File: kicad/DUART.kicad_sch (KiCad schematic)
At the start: 1 part

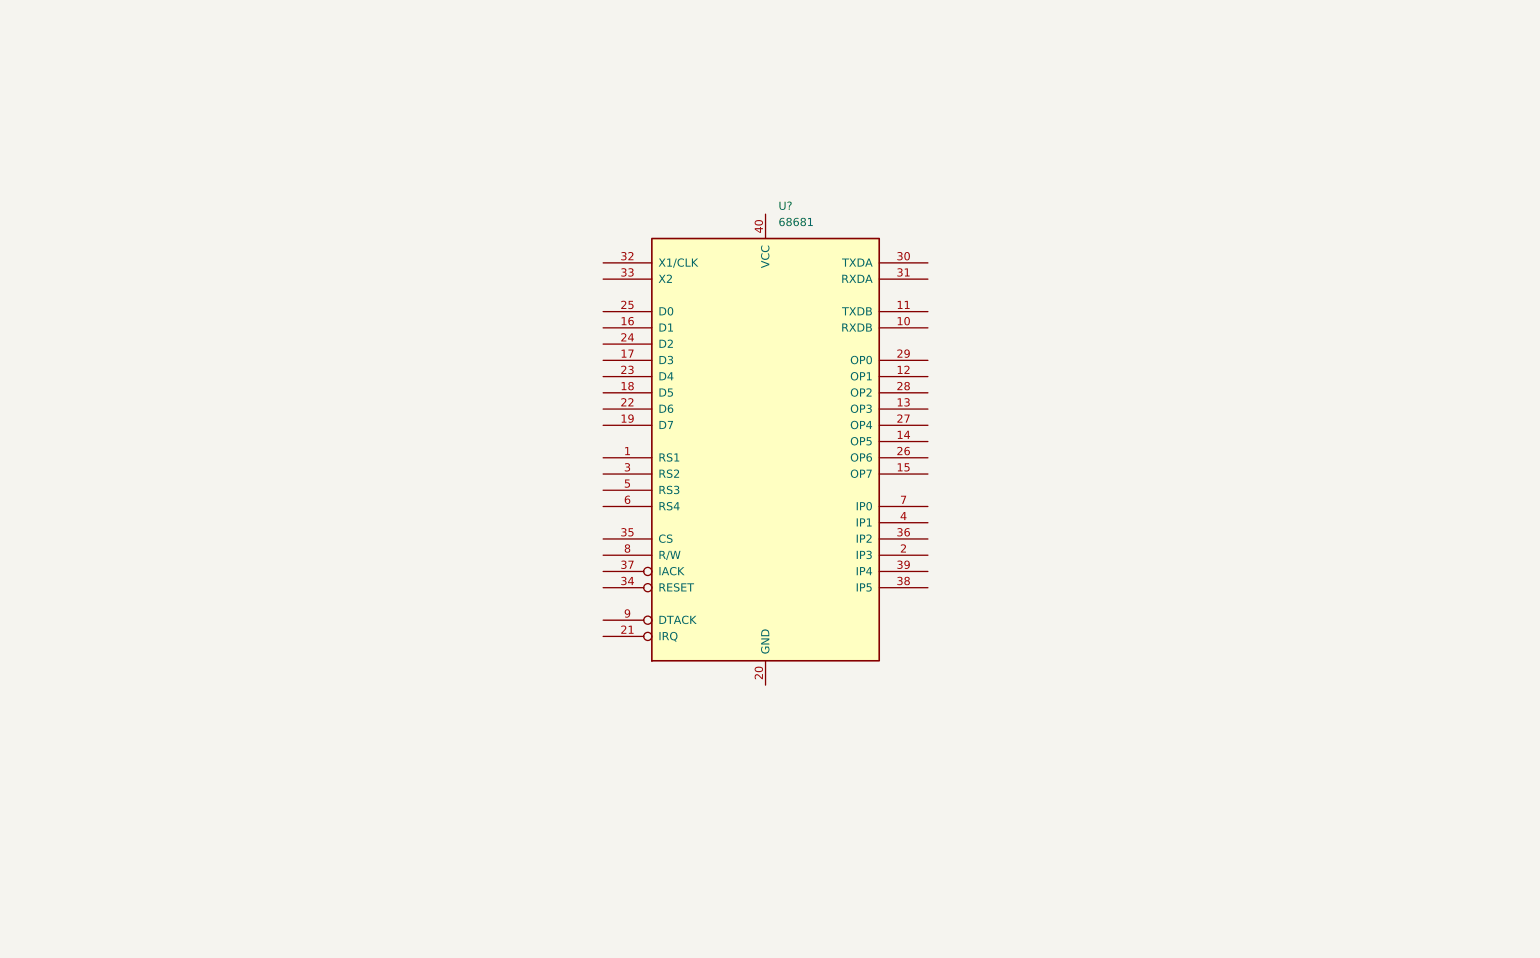
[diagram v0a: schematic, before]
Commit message: Lot of stuff. Memmory decoder in GAL Added README for Digital Updated sketch for Arduino
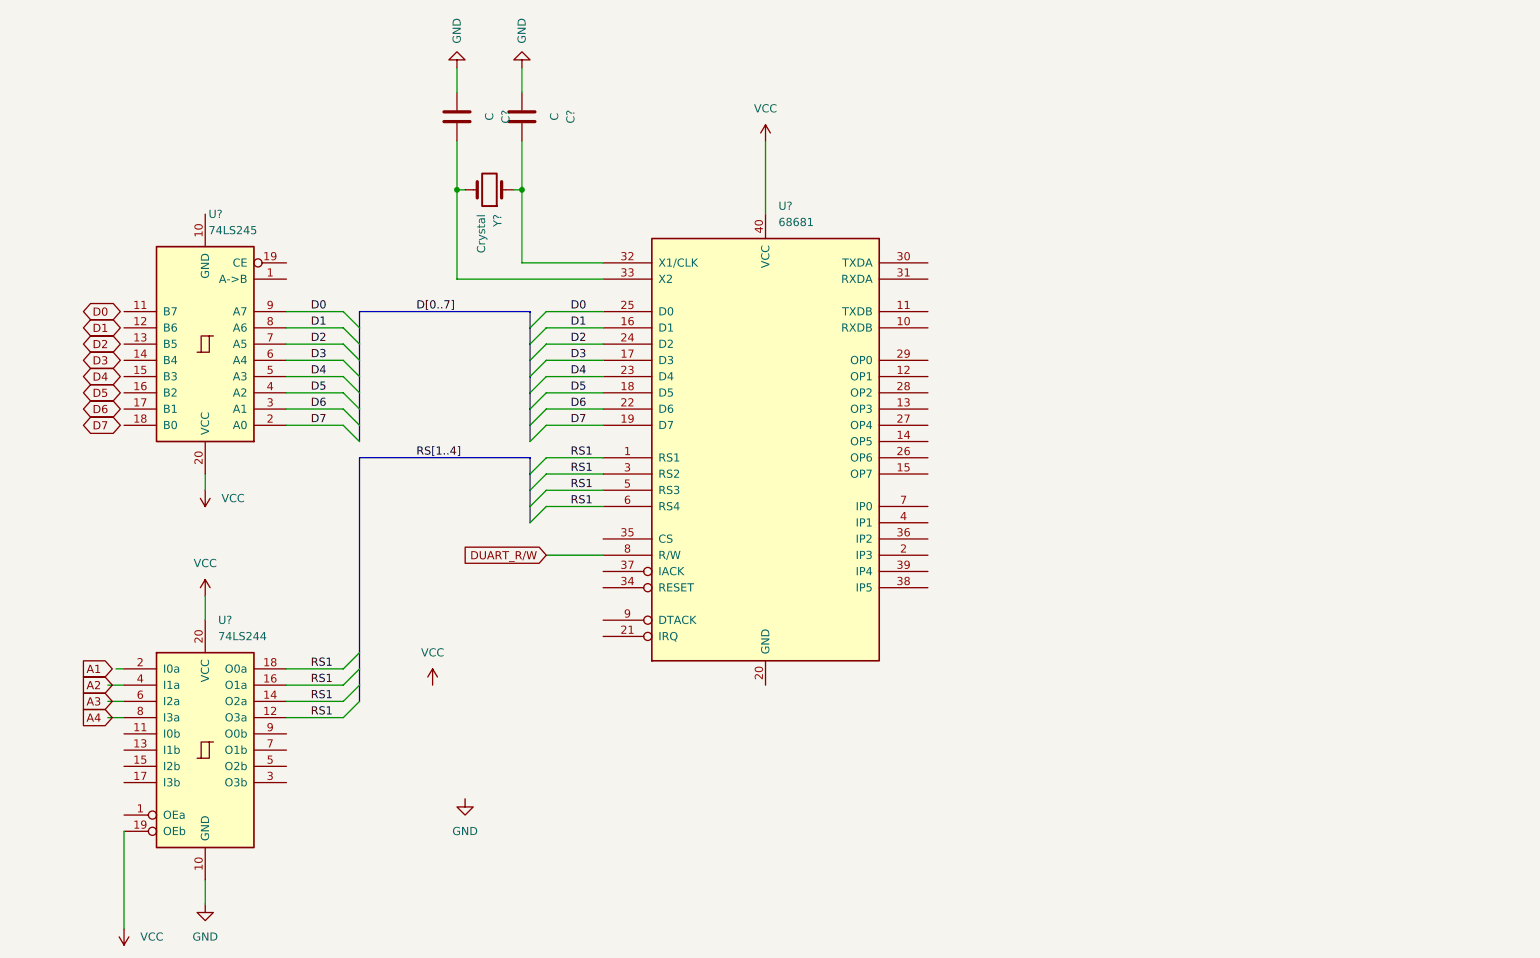
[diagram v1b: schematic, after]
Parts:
- added C? (x2): C, symbol Device:C
- added U?: 74LS245, symbol 74xx:74LS245
- added U?: 74LS244, symbol 74xx:74LS244
- added Y?: Crystal, symbol Device:Crystal
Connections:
- net RS1: now reaches U?.1 (RS1)
- net RS1: now also U?.3 (RS2), U?.5 (RS3), U?.6 (RS4), U?.12 (O3a), U?.14 (O2a), U?.16 (O1a), U?.18 (O0a)
- net D1: now reaches U?.16 (D1)
- net D1: now also U?.8 (A6)
- net D3: now reaches U?.17 (D3)
- net D3: now also U?.6 (A4)
- net D5: now reaches U?.18 (D5)
- net D5: now also U?.4 (A2)
- net D7: now reaches U?.19 (D7)
- net D7: now also U?.2 (A0)
- net D6: now reaches U?.22 (D6)
- net D6: now also U?.3 (A1)
- net D4: now reaches U?.23 (D4)
- net D4: now also U?.5 (A3)
- net D2: now reaches U?.24 (D2)
- net D2: now also U?.7 (A5)
- net D0: now reaches U?.25 (D0)
- net D0: now also U?.9 (A7)
- net at U?.32 (X1/CLK): now also C?.2, Y?.1
- net at U?.33 (X2): now also C?.2, Y?.2
- net VCC: now reaches U?.40 (VCC)
- net VCC: now also U?.19 (OEb), U?.20 (VCC), U?.20 (VCC)
- net DUART_R/W: now reaches U?.8 (R/W)
- new net GND: C?.1, C?.1, U?.10 (GND)

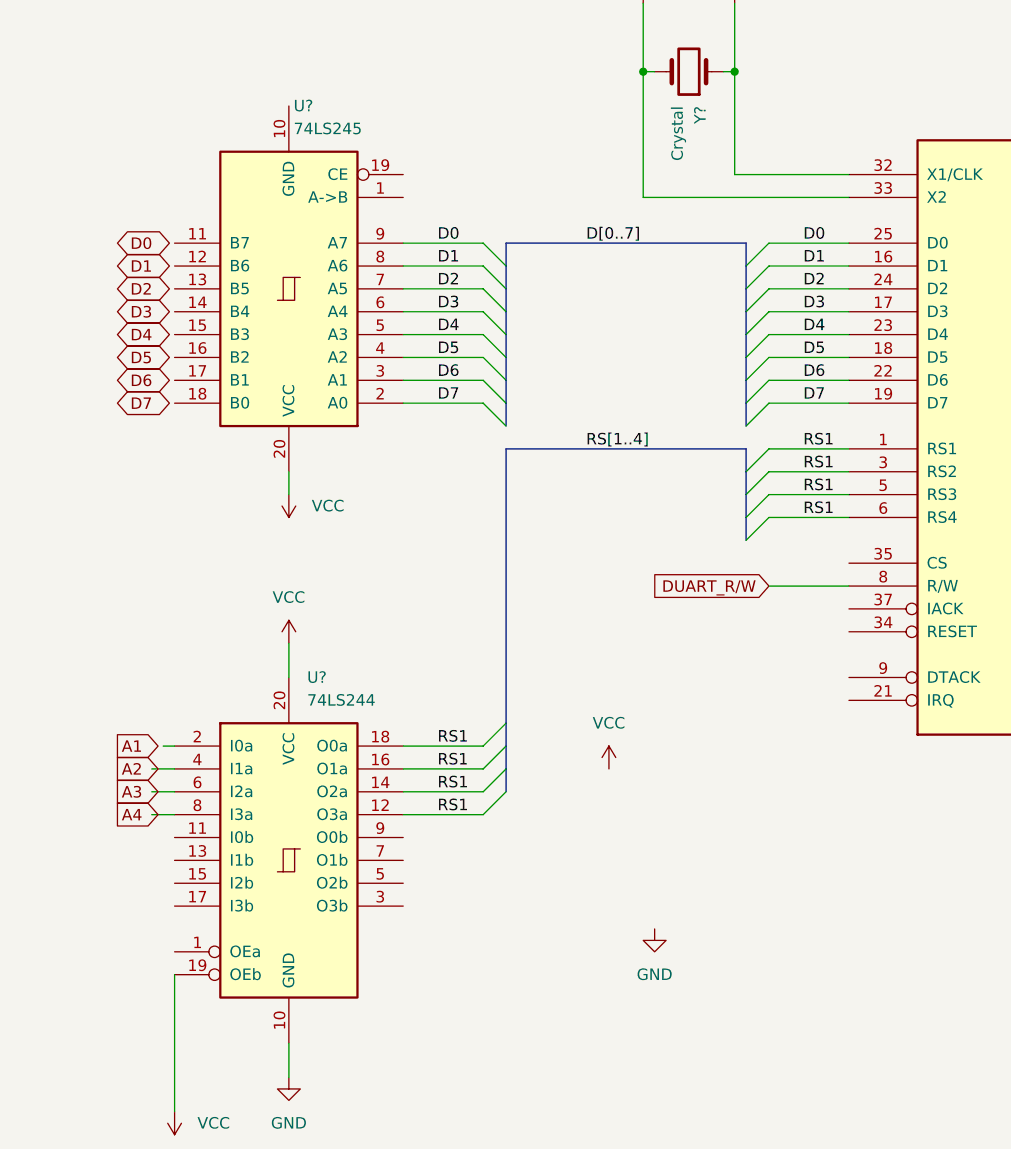
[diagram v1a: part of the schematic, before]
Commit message: KiCad updates
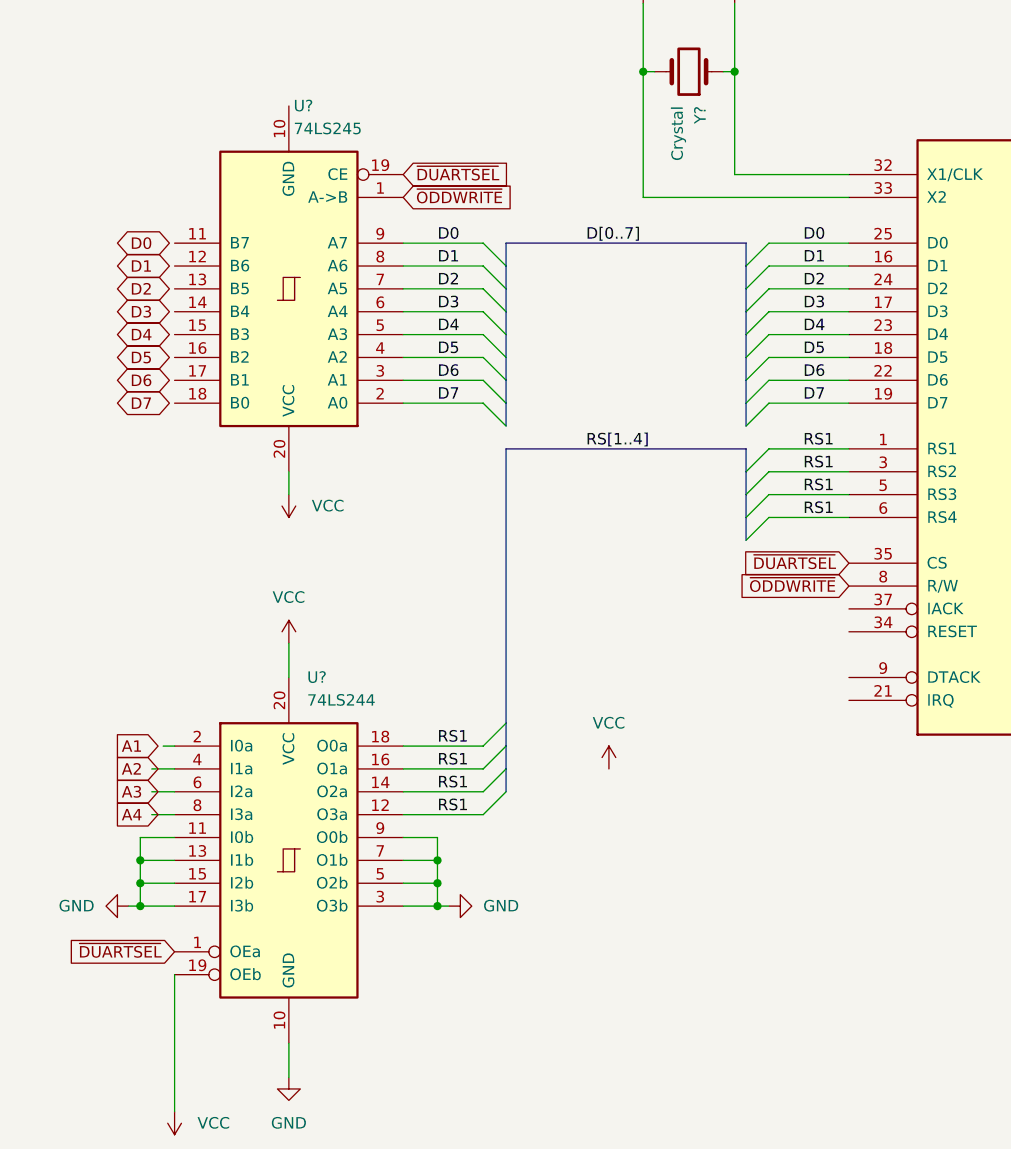
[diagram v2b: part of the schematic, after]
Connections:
- net DUART_R/W is gone; now on net ~{ODDWRITE}: U?.8 (R/W)
- net GND: now also U?.11 (I0b), U?.13 (I1b), U?.15 (I2b), U?.17 (I3b), U?.3 (O3b), U?.5 (O2b), U?.7 (O1b), U?.9 (O0b)
- net ~{DUARTSEL}: now reaches U?.35 (CS)
- net ~{DUARTSEL}: now also U?.1 (OEa), U?.19 (CE)
- net ~{ODDWRITE}: now reaches U?.1 (A->B)
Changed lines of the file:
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@@
 (kicad_sch (version 20211123) (generator eeschema)
   (paper "A4")
+  (junction (at 38.1 134.62) (diameter 0) (color 0 0 0 0)
+  )
+  (junction (at 38.1 132.08) (diameter 0) (color 0 0 0 0)
+  )
+  (junction (at 71.12 132.08) (diameter 0) (color 0 0 0 0)
+  )
   (junction (at 93.98 44.45) (diameter 0) (color 0 0 0 0)
   )
+  (junction (at 38.1 137.16) (diameter 0) (color 0 0 0 0)
+  )
   (junction (at 104.14 44.45) (diameter 0) (color 0 0 0 0)
   )
+  (junction (at 71.12 134.62) (diameter 0) (color 0 0 0 0)
+  )
+  (junction (at 71.12 137.16) (diameter 0) (color 0 0 0 0)
+  )
   (bus_entry (at 105.41 71.12) (size 2.54 -2.54)
     (stroke (width 0) (type default) (color 0 0 0 0))
@@
     (stroke (width 0) (type default) (color 0 0 0 0))
   )
+  (wire (pts (xy 67.31 137.16) (xy 71.12 137.16))
+    (stroke (width 0) (type default) (color 0 0 0 0))
+  )
   (bus (pts (xy 105.41 93.98) (xy 105.41 91.44))
     (stroke (width 0) (type default) (color 0 0 0 0))
   )
+  (wire (pts (xy 71.12 134.62) (xy 71.12 137.16))
+    (stroke (width 0) (type default) (color 0 0 0 0))
+  )
+  (wire (pts (xy 71.12 129.54) (xy 71.12 132.08))
+    (stroke (width 0) (type default) (color 0 0 0 0))
+  )
   (wire (pts (xy 107.95 66.04) (xy 116.84 66.04))
     (stroke (width 0) (type default) (color 0 0 0 0))
@@
     (stroke (width 0) (type default) (color 0 0 0 0))
   )
+  (wire (pts (xy 67.31 134.62) (xy 71.12 134.62))
+    (stroke (width 0) (type default) (color 0 0 0 0))
+  )
   (bus (pts (xy 105.41 73.66) (xy 105.41 76.2))
     (stroke (width 0) (type default) (color 0 0 0 0))
@@
     (stroke (width 0) (type default) (color 0 0 0 0))
   )
+  (wire (pts (xy 67.31 132.08) (xy 71.12 132.08))
+    (stroke (width 0) (type default) (color 0 0 0 0))
+  )
+  (wire (pts (xy 71.12 137.16) (xy 72.39 137.16))
+    (stroke (width 0) (type default) (color 0 0 0 0))
+  )
   (bus (pts (xy 105.41 68.58) (xy 105.41 71.12))
     (stroke (width 0) (type default) (color 0 0 0 0))
@@
     (stroke (width 0) (type default) (color 0 0 0 0))
   )
-  (wire (pts (xy 107.95 101.6) (xy 116.84 101.6))
+  (wire (pts (xy 38.1 134.62) (xy 38.1 137.16))
     (stroke (width 0) (type default) (color 0 0 0 0))
   )
@@
     (stroke (width 0) (type default) (color 0 0 0 0))
   )
+  (wire (pts (xy 36.83 137.16) (xy 38.1 137.16))
+    (stroke (width 0) (type default) (color 0 0 0 0))
+  )
   (bus (pts (xy 105.41 71.12) (xy 105.41 73.66))
     (stroke (width 0) (type default) (color 0 0 0 0))
@@
     (stroke (width 0) (type default) (color 0 0 0 0))
   )
+  (wire (pts (xy 38.1 134.62) (xy 41.91 134.62))
+    (stroke (width 0) (type default) (color 0 0 0 0))
+  )
   (wire (pts (xy 104.14 25.4) (xy 104.14 29.21))
     (stroke (width 0) (type default) (color 0 0 0 0))
@@
     (stroke (width 0) (type default) (color 0 0 0 0))
   )
+  (wire (pts (xy 67.31 129.54) (xy 71.12 129.54))
+    (stroke (width 0) (type default) (color 0 0 0 0))
+  )
   (bus (pts (xy 78.74 121.92) (xy 78.74 124.46))
     (stroke (width 0) (type default) (color 0 0 0 0))
   )
+  (wire (pts (xy 38.1 137.16) (xy 41.91 137.16))
+    (stroke (width 0) (type default) (color 0 0 0 0))
+  )
   (wire (pts (xy 93.98 44.45) (xy 93.98 58.42))
     (stroke (width 0) (type default) (color 0 0 0 0))
   )
+  (wire (pts (xy 38.1 132.08) (xy 41.91 132.08))
+    (stroke (width 0) (type default) (color 0 0 0 0))
+  )
   (bus (pts (xy 78.74 68.58) (xy 78.74 66.04))
     (stroke (width 0) (type default) (color 0 0 0 0))
   )
+  (wire (pts (xy 38.1 132.08) (xy 38.1 134.62))
+    (stroke (width 0) (type default) (color 0 0 0 0))
+  )
   (wire (pts (xy 104.14 44.45) (xy 104.14 55.88))
     (stroke (width 0) (type default) (color 0 0 0 0))
@@
     (stroke (width 0) (type default) (color 0 0 0 0))
   )
+  (wire (pts (xy 38.1 129.54) (xy 38.1 132.08))
+    (stroke (width 0) (type default) (color 0 0 0 0))
+  )
   (wire (pts (xy 107.95 76.2) (xy 116.84 76.2))
     (stroke (width 0) (type default) (color 0 0 0 0))
   )
+  (wire (pts (xy 41.91 129.54) (xy 38.1 129.54))
+    (stroke (width 0) (type default) (color 0 0 0 0))
+  )
   (bus (pts (xy 105.41 96.52) (xy 105.41 93.98))
     (stroke (width 0) (type default) (color 0 0 0 0))
@@
     (stroke (width 0) (type default) (color 0 0 0 0))
   )
+  (wire (pts (xy 71.12 132.08) (xy 71.12 134.62))
+    (stroke (width 0) (type default) (color 0 0 0 0))
+  )
   (wire (pts (xy 104.14 44.45) (xy 102.87 44.45))
     (stroke (width 0) (type default) (color 0 0 0 0))
@@
     )
   )
-  (global_label "DUART_R{slash}W" (shape input) (at 107.95 101.6 180) (fields_autoplaced)
+  (global_label "~{DUARTSEL}" (shape input) (at 116.84 99.06 180) (fields_autoplaced)
     (effects (font (size 1.27 1.27)) (justify right))
-    (property "Intersheet References" "${INTERSHEET_REFS}" (id 0) (at 94.5907 101.5206 0)
+    (property "Intersheet References" "${INTERSHEET_REFS}" (id 0) (at 105.1136 99.1394 0)
       (effects (font (size 1.27 1.27)) (justify right) hide)
     )
@@
     )
   )
+  (global_label "~{ODDWRITE}" (shape input) (at 116.84 101.6 180) (fields_autoplaced)
+    (effects (font (size 1.27 1.27)) (justify right))
+    (property "Intersheet References" "${INTERSHEET_REFS}" (id 0) (at 105.1136 101.5206 0)
+      (effects (font (size 1.27 1.27)) (justify right) hide)
+    )
+  )
   (global_label "D6" (shape bidirectional) (at 35.56 78.74 0) (fields_autoplaced)
     (effects (font (size 1.27 1.27)) (justify left))
@@
     )
   )
+  (global_label "~{DUARTSEL}" (shape input) (at 41.91 142.24 180) (fields_autoplaced)
+    (effects (font (size 1.27 1.27)) (justify right))
+    (property "Intersheet References" "${INTERSHEET_REFS}" (id 0) (at 30.1836 142.3194 0)
+      (effects (font (size 1.27 1.27)) (justify right) hide)
+    )
+  )
+  (global_label "~{DUARTSEL}" (shape input) (at 67.31 55.88 0) (fields_autoplaced)
+    (effects (font (size 1.27 1.27)) (justify left))
+    (property "Intersheet References" "${INTERSHEET_REFS}" (id 0) (at 79.0364 55.8006 0)
+      (effects (font (size 1.27 1.27)) (justify left) hide)
+    )
+  )
   (global_label "A4" (shape output) (at 35.56 127 0) (fields_autoplaced)
     (effects (font (size 1.27 1.27)) (justify left))
     (property "Intersheet References" "${INTERSHEET_REFS}" (id 0) (at 40.2712 126.9206 0)
+      (effects (font (size 1.27 1.27)) (justify left) hide)
+    )
+  )
+  (global_label "~{ODDWRITE}" (shape input) (at 67.31 58.42 0) (fields_autoplaced)
+    (effects (font (size 1.27 1.27)) (justify left))
+    (property "Intersheet References" "${INTERSHEET_REFS}" (id 0) (at 79.0364 58.4994 0)
       (effects (font (size 1.27 1.27)) (justify left) hide)
     )
@@
     (pin "1")
   )
-  (symbol (lib_id "power:GND") (at 95.25 139.7 0) (unit 1)
-    (in_bom yes) (on_board yes) (fields_autoplaced)
-    (property "Reference" "#PWR?" (id 0) (at 95.25 146.05 0)
-      (effects (font (size 1.27 1.27)) hide)
-    )
-    (property "Value" "GND" (id 1) (at 95.25 144.78 0))
-    (property "Footprint" "" (id 2) (at 95.25 139.7 0)
-      (effects (font (size 1.27 1.27)) hide)
-    )
-    (property "Datasheet" "" (id 3) (at 95.25 139.7 0)
+  (symbol (lib_id "power:GND") (at 36.83 137.16 270) (unit 1)
+    (in_bom yes) (on_board yes) (fields_autoplaced)
+    (property "Reference" "#PWR?" (id 0) (at 30.48 137.16 0)
+      (effects (font (size 1.27 1.27)) hide)
+    )
+    (property "Value" "GND" (id 1) (at 33.02 137.1599 90)
+      (effects (font (size 1.27 1.27)) (justify right))
+    )
+    (property "Footprint" "" (id 2) (at 36.83 137.16 0)
+      (effects (font (size 1.27 1.27)) hide)
+    )
+    (property "Datasheet" "" (id 3) (at 36.83 137.16 0)
       (effects (font (size 1.27 1.27)) hide)
     )
@@
       (effects (font (size 1.27 1.27)) hide)
     )
+    (pin "1")
+  )
+  (symbol (lib_id "power:GND") (at 72.39 137.16 90) (unit 1)
+    (in_bom yes) (on_board yes) (fields_autoplaced)
+    (property "Reference" "#PWR?" (id 0) (at 78.74 137.16 0)
+      (effects (font (size 1.27 1.27)) hide)
+    )
+    (property "Value" "GND" (id 1) (at 76.2 137.1599 90)
+      (effects (font (size 1.27 1.27)) (justify right))
+    )
+    (property "Footprint" "" (id 2) (at 72.39 137.16 0)
+      (effects (font (size 1.27 1.27)) hide)
+    )
+    (property "Datasheet" "" (id 3) (at 72.39 137.16 0)
+      (effects (font (size 1.27 1.27)) hide)
+    )
